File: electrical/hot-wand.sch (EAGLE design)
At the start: 202 parts, among them IC1 12V R-78K12-2.0, IC2 3V3 R-78K3.3, Q1 STP19NF20, Q2 IRF510, Q3 BC846B, Q4 SIS862ADN-T1-GE3, Q5 SIS862ADN-T1-GE3, Q6 DMTH64M2LPDWQ-13, Q7 SIS862ADN-T1-GE3, Q8 2N7002K, Q9 G3404, SW1 SW-TACT-SIDE, U1 TPS54560DDA, U2 1EDN8511BXUSA1, U3 STM32F042F6P6, U4 SSD1306-4PIN-0.91N-VERT, U5 INA138, U6 LM74810QDRRRQ1, U7 AP53781, Y1 27.12 MHz 10pF

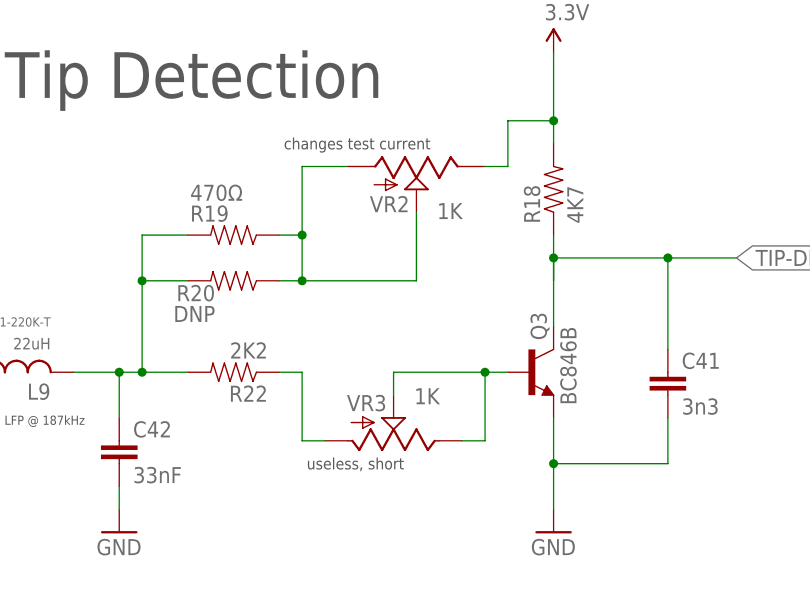
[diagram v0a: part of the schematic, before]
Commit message: pcb assembly problems being addressed
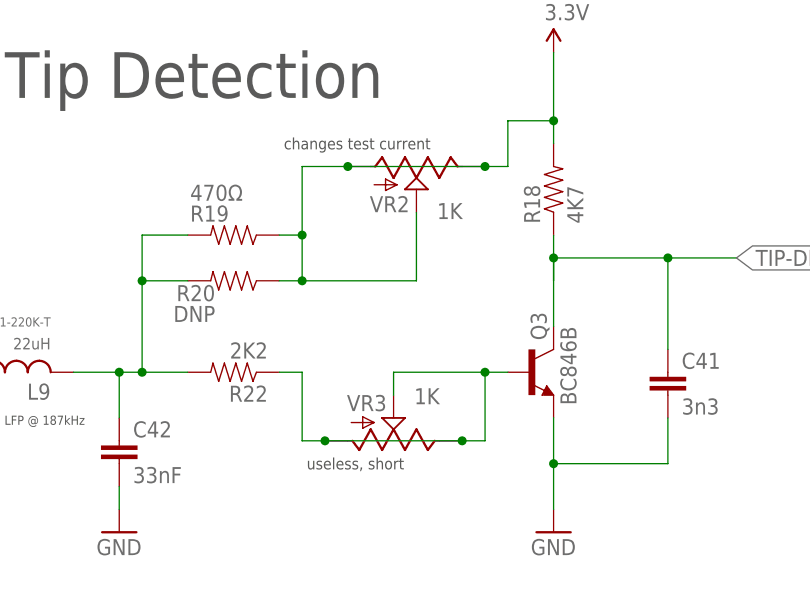
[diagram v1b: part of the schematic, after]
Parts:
- C10, C11, C12, C13, C14, C15, C16, C17, C18, C19, C20, C21, C22, C23, C24, C25, C26, C27, C28, C29, C30, C31, C32, C33, C37, C38, C39, C40, C9: device hot-wand:CAP0805 -> hot-wand:CAP0805-L
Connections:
- removed net N$45: R19.1, R20.1, VR2.A, VR2.S
- removed net N$8: R22.1, VR3.A
- net 3.3V: now also R19.1, R20.1, VR2.A, VR2.S
- net Q3-VB: now also R22.1, VR3.A
